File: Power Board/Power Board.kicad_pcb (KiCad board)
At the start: 2 copper layers, 55 x 70 mm, 147 parts, among them J1 Conn_02x07_Odd_Even, J2 Screw_Terminal_01x06, J3 Conn_01x03, J4 Conn_01x02, J5 Conn_02x03_Odd_Even, Q1 SI7157DP, Q2 SI7157DP, Q3 SI7157DP, Q4 SI7157DP, Q5 SI7157DP, Q6 SI7157DP, Q7 DMG2305UX, U1 LTC4417CGN, U10 LTC4150, U11 ATxmega32E5-AU, U2 TPS564208DDCT, U3 LTC3130-1, U4 LMR62014XMF, U5 TPS22810, U6 BQ2057WSNTR, U7 BQ29209DRBT, U8 LT6700CS6-1, U9 STS8C5H30L

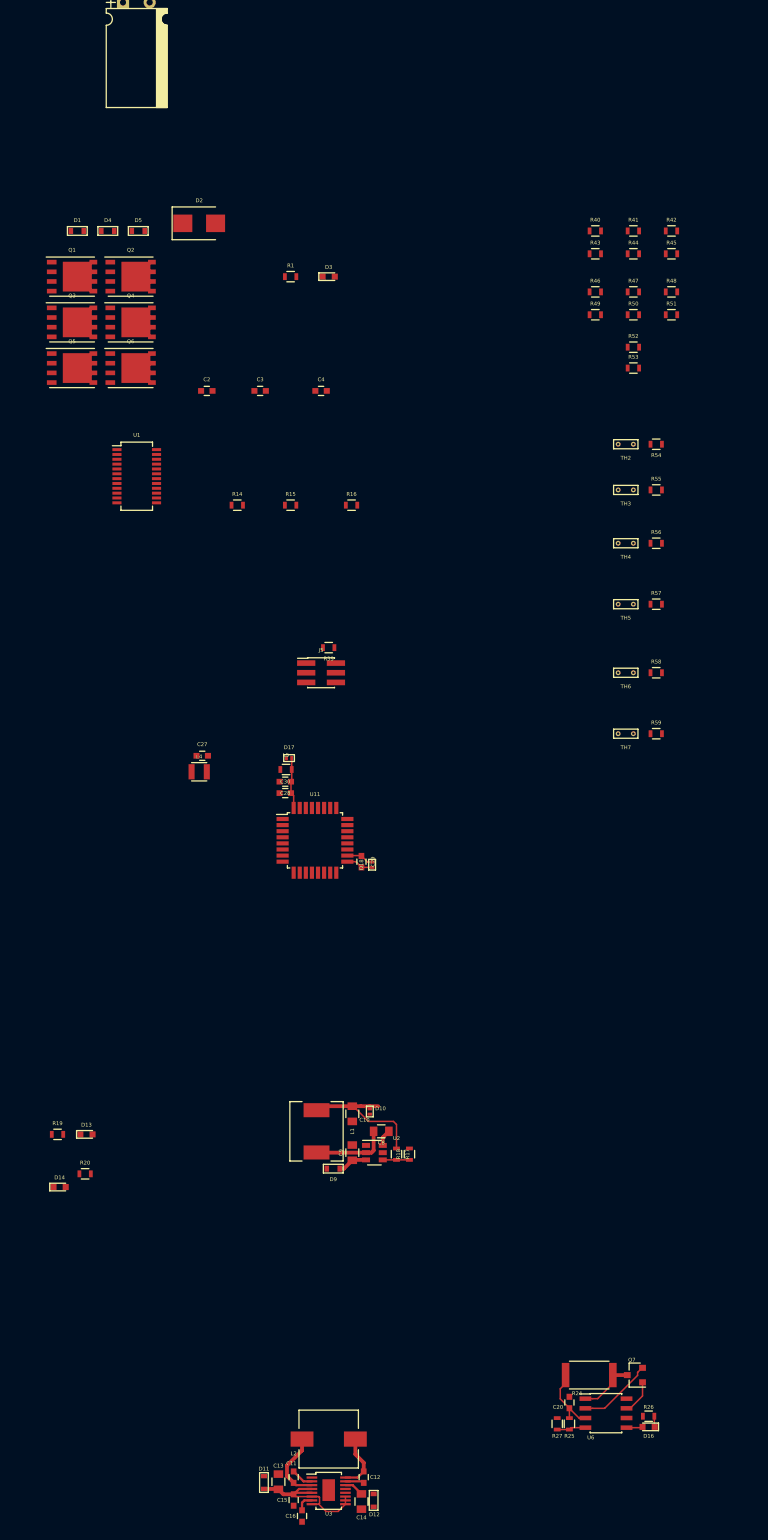
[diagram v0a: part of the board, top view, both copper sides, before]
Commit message: More changes
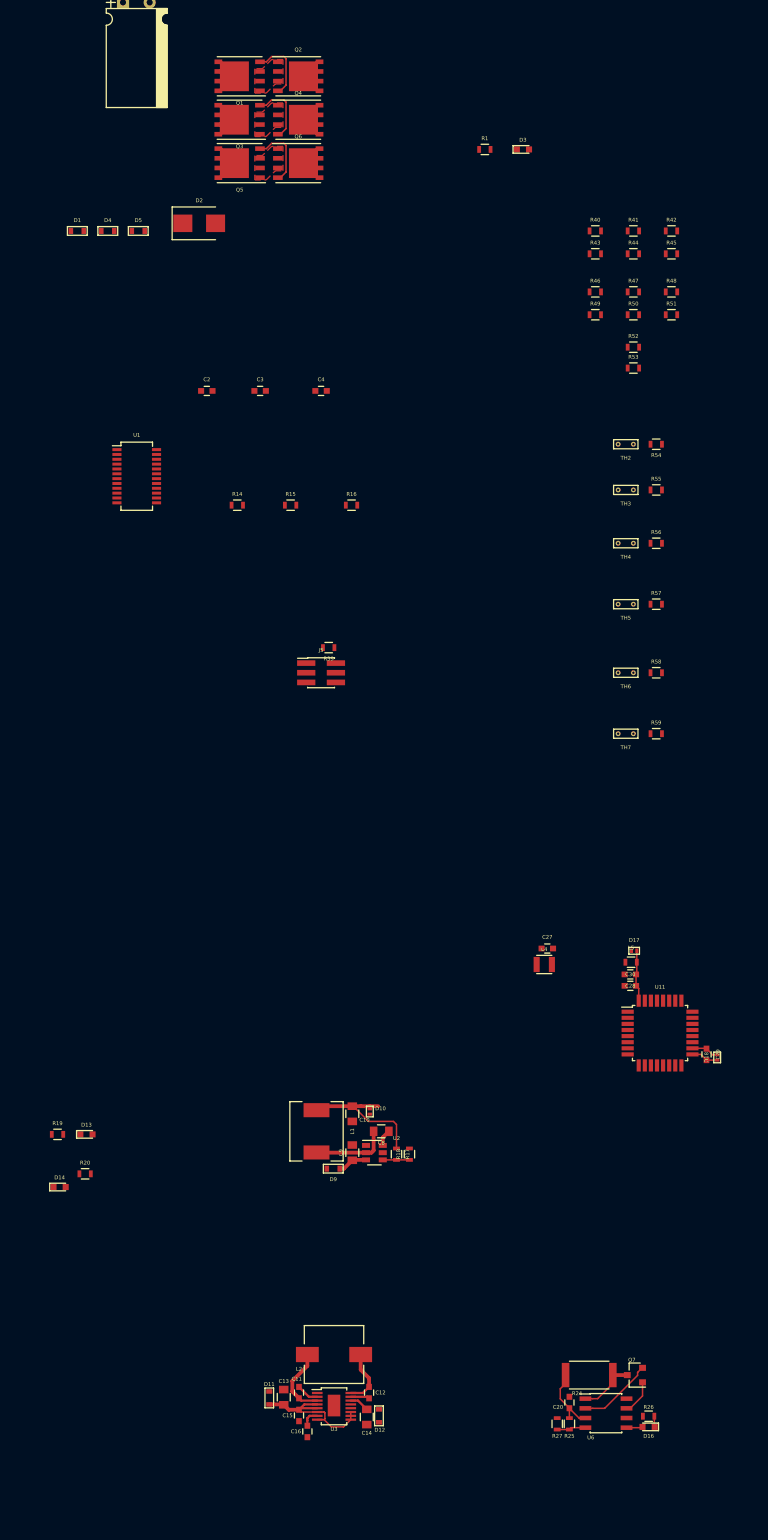
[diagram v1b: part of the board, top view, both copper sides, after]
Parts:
- moved C28 51.9 mm to (368.7, 124.9)
- moved C29 51.9 mm to (378.7, 135.4)
- moved C30 51.9 mm to (368.7, 126.4)
- moved D17 51.9 mm to (369.2, 121.8)
- moved D18 51.9 mm to (380.1, 135.8)
- moved L4 51.9 mm to (357.4, 123.6)
- moved U11 51.9 mm to (372.6, 132.6)
- moved C27 51.9 mm to (357.8, 121.5)
- moved L5 51.9 mm to (368.8, 123.3)
- moved Q5 34.8 mm to (317.4, 18.4), turned to 180 degrees
- moved Q6 34.8 mm to (325.1, 18.4)
- moved Q4 34.5 mm to (325.1, 12.7)
- moved Q3 34.5 mm to (317.4, 12.7), turned to 180 degrees
- moved Q1 34.3 mm to (317.4, 7.03), turned to 180 degrees
- moved Q2 34.3 mm to (325.1, 7.03)
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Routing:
- net Net-(Q3-Pad2): track 0.00 -> 8.69 mm
- net Net-(Q5-Pad2): track 0.00 -> 8.68 mm
- net Net-(Q1-Pad2): track 0.00 -> 8.68 mm
- added copper zone on F.Cu, net Net-(C2-Pad1)
- added copper zone on F.Cu, net Net-(C3-Pad1)
- added copper zone on F.Cu, net Net-(C4-Pad1)
